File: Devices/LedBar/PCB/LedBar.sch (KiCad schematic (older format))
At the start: 6 parts

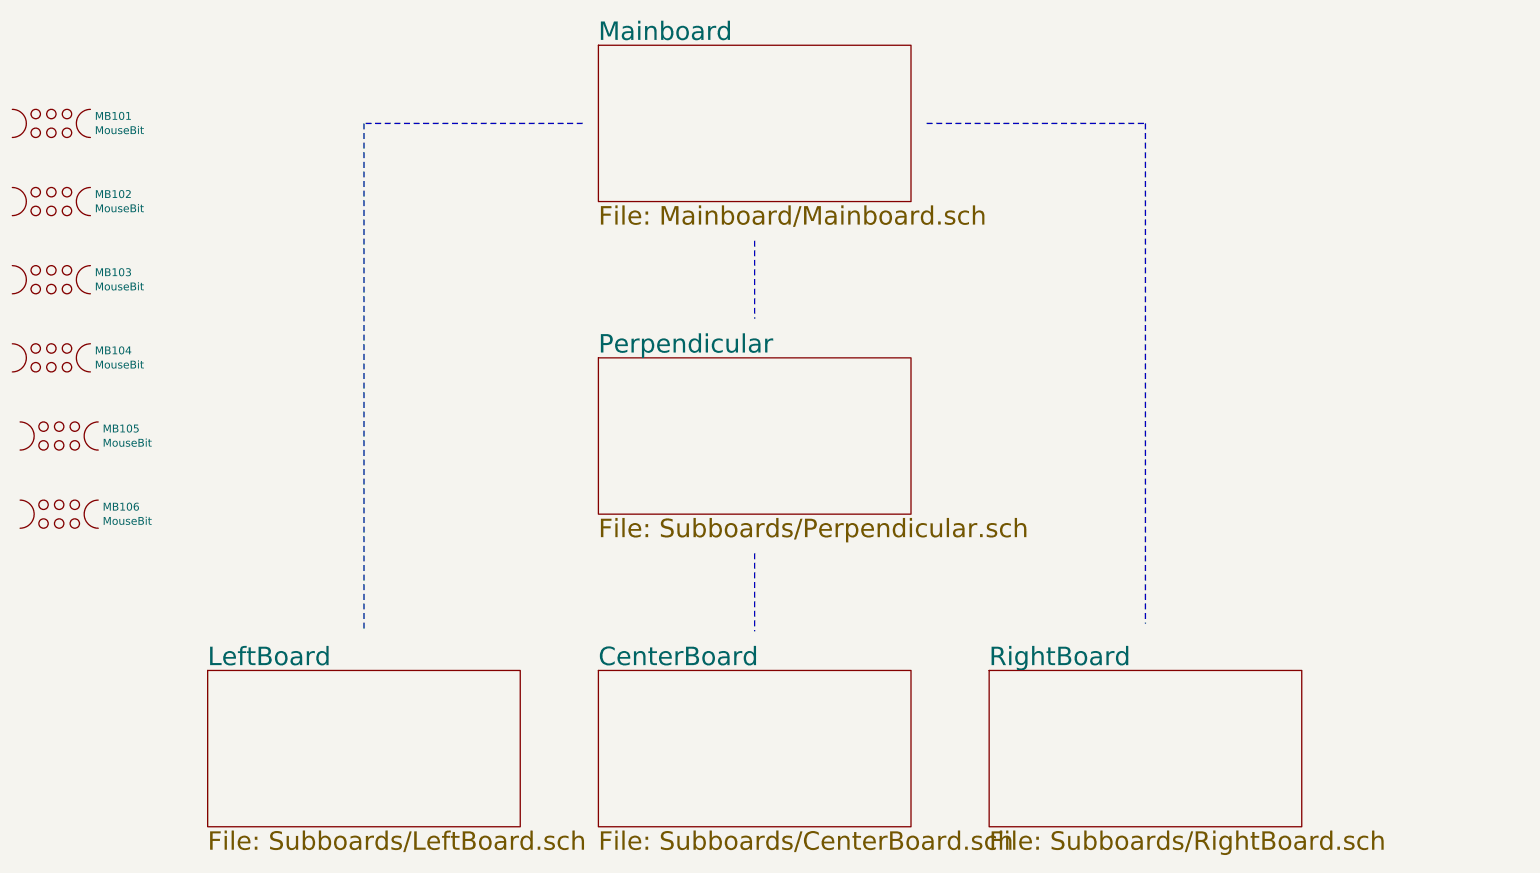
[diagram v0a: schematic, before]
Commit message: Releasing RGBW-LEDBar v2.0
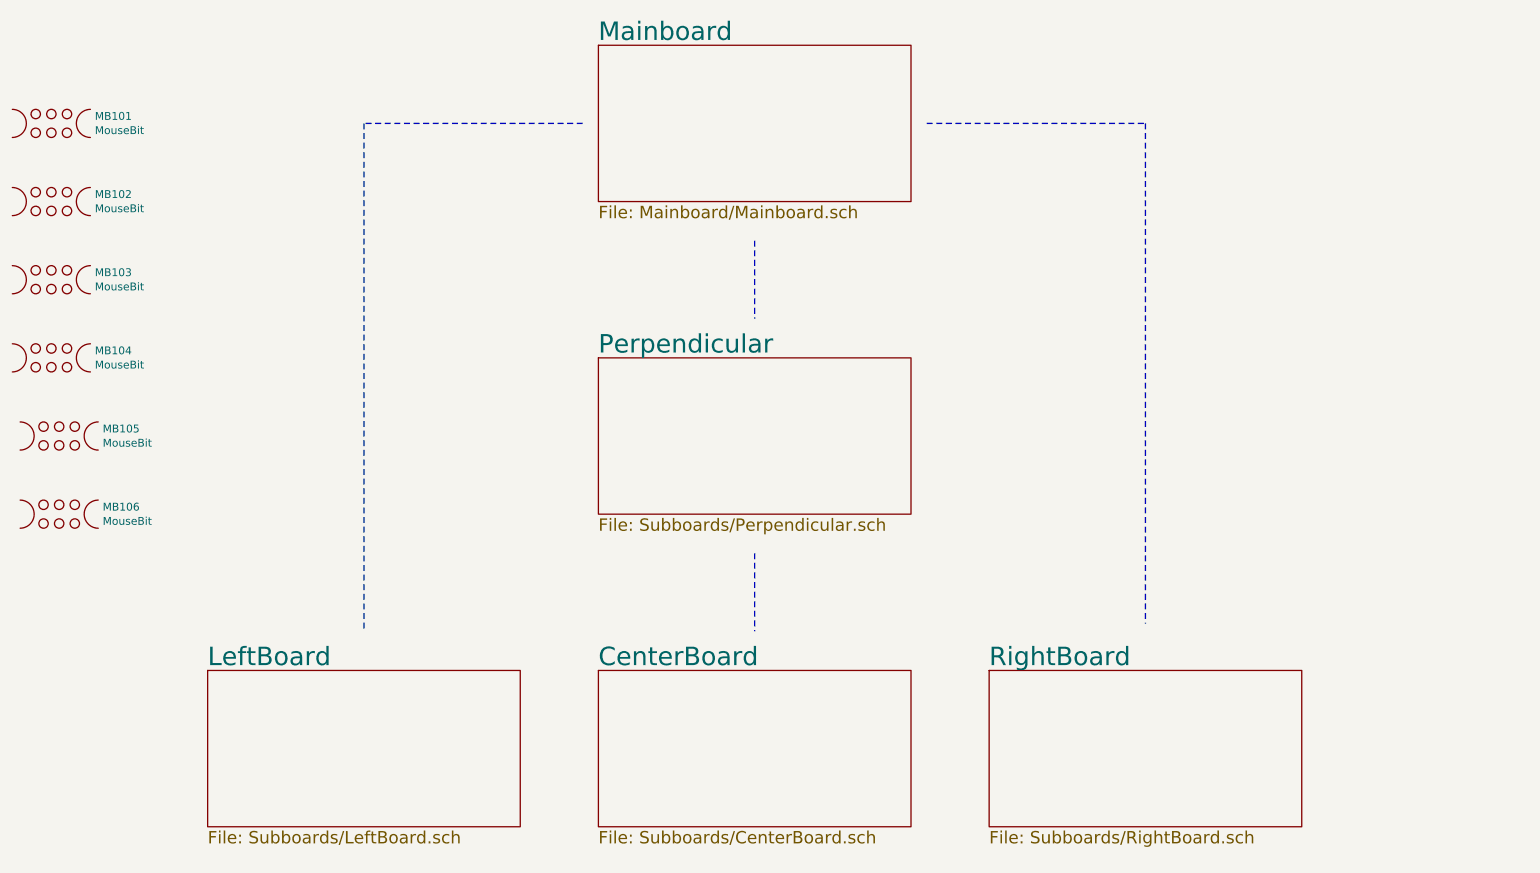
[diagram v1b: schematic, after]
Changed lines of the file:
@@
 Sheet 1 13
 Title "LedBar - MainBoard"
-Date "2022-06-26"
-Rev "1.0"
+Date "2022-12-06"
+Rev "2.0"
 Comp "Roel Drost"
 Comment1 "GNU General Public License v3.0"
@@
 U 617A8CB5
 F0 "Mainboard" 118
-F1 "Mainboard/Mainboard.sch" 118
+F1 "Mainboard/Mainboard.sch" 79
 $EndSheet
 $Sheet
@@
 U 618804D0
 F0 "LeftBoard" 118
-F1 "Subboards/LeftBoard.sch" 118
+F1 "Subboards/LeftBoard.sch" 79
 $EndSheet
 $Sheet
@@
 U 6188050F
 F0 "CenterBoard" 118
-F1 "Subboards/CenterBoard.sch" 118
+F1 "Subboards/CenterBoard.sch" 79
 $EndSheet
 $Sheet
@@
 U 6188055C
 F0 "RightBoard" 118
-F1 "Subboards/RightBoard.sch" 118
+F1 "Subboards/RightBoard.sch" 79
 $EndSheet
 $Sheet
@@
 U 6187FE9B
 F0 "Perpendicular" 118
-F1 "Subboards/Perpendicular.sch" 118
+F1 "Subboards/Perpendicular.sch" 79
 $EndSheet
 $Comp
